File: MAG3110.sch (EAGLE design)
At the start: 4 parts

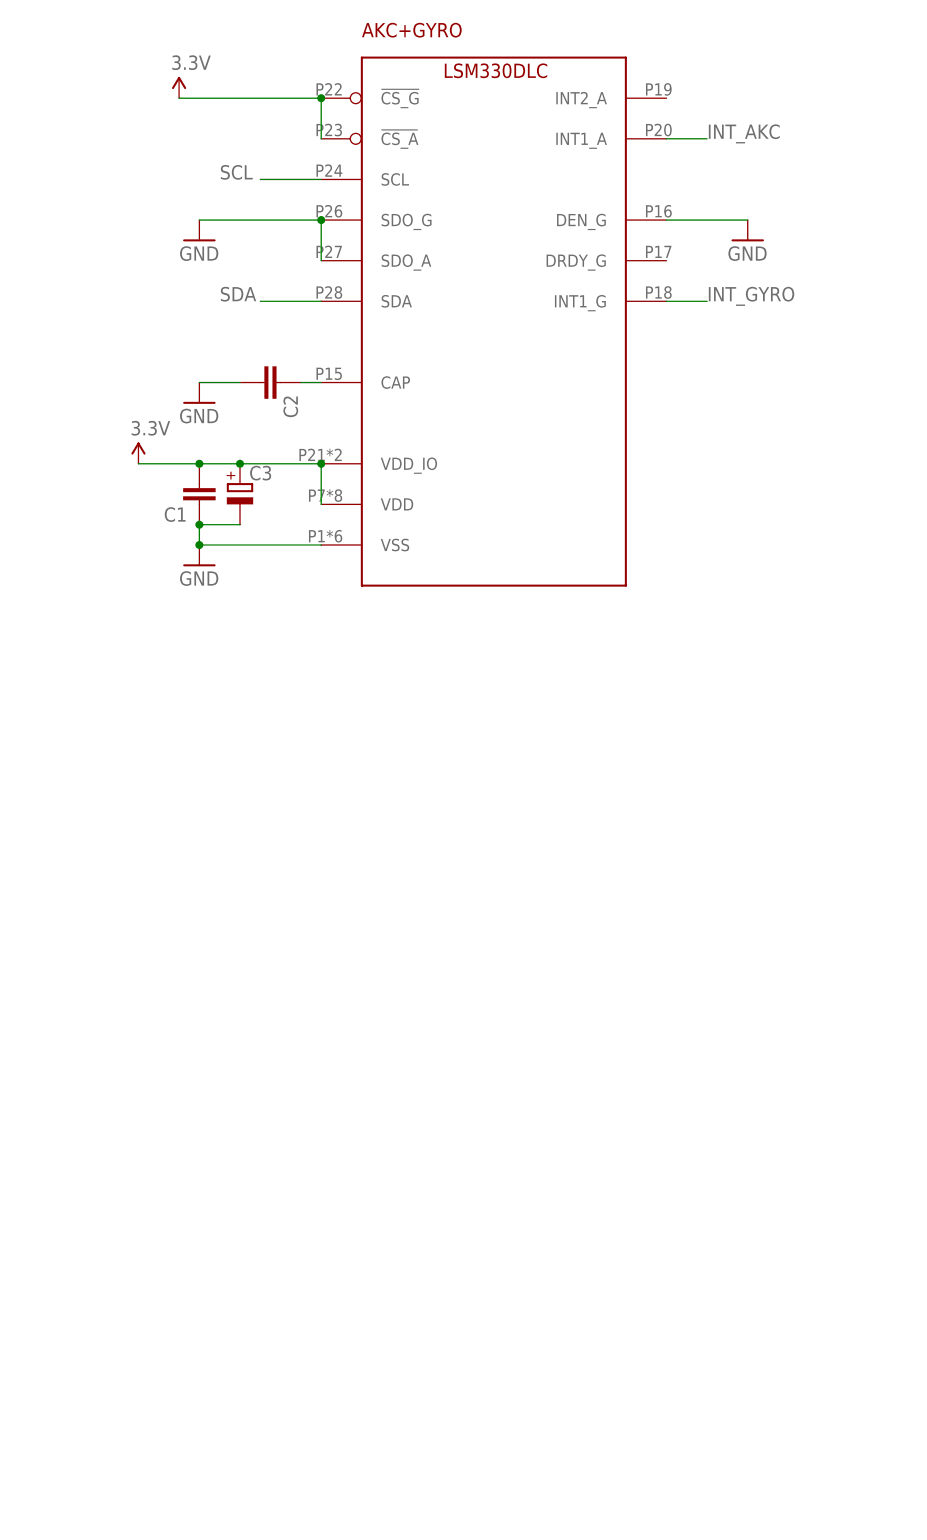
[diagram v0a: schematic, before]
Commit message: porzadki w plikach
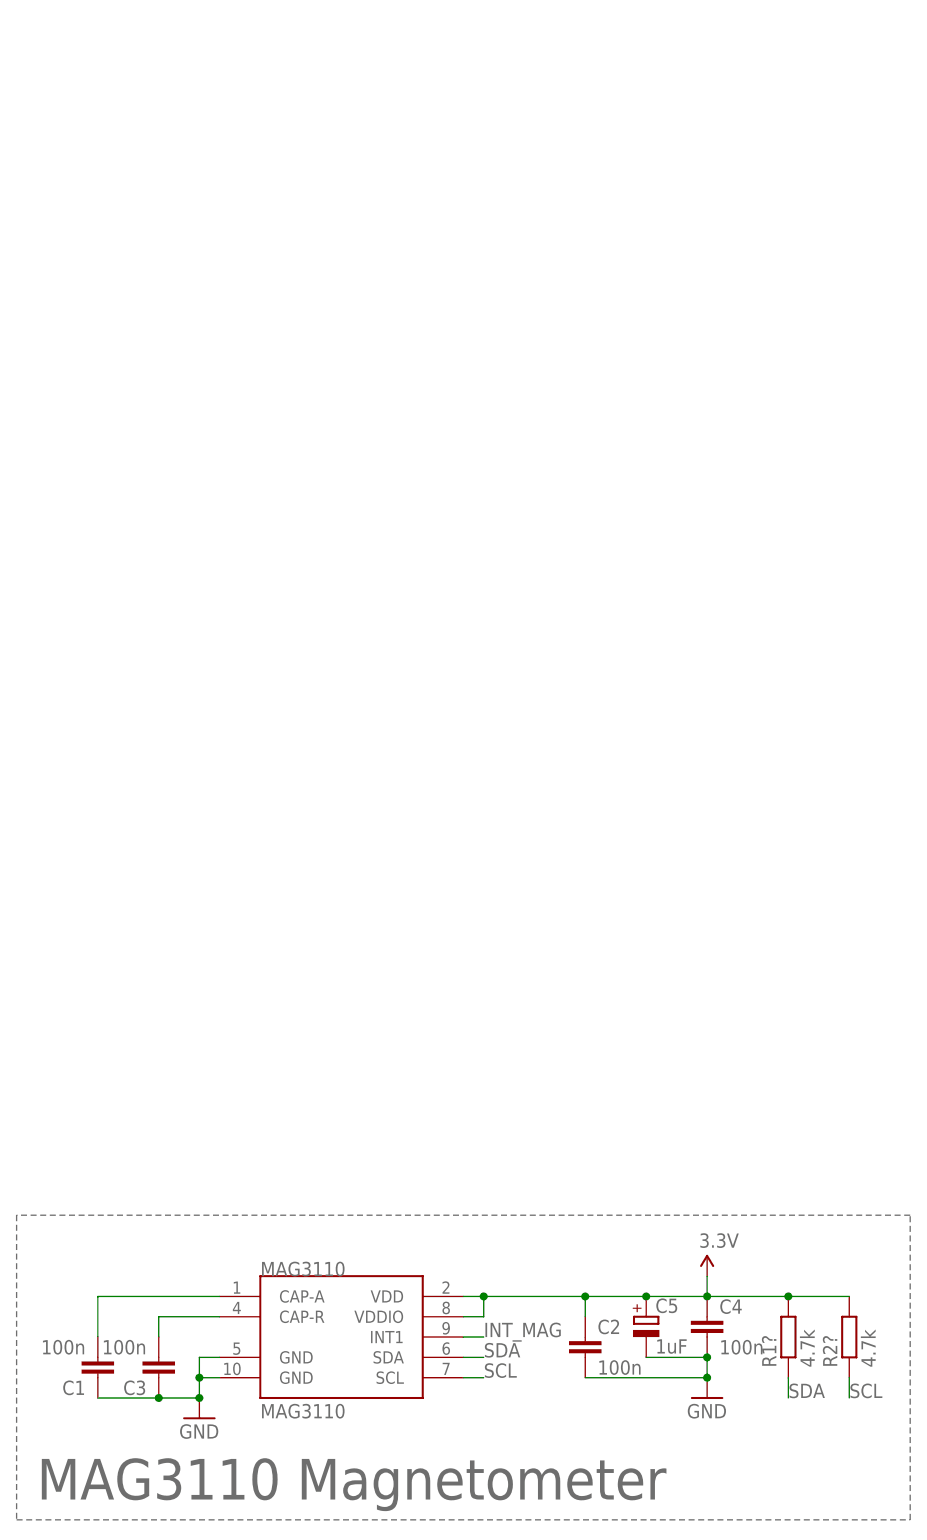
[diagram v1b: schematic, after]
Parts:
- removed AKC+GYRO: LSM330DLC, sensors-akc_zyr:LSM330DLC
- added C4: 100n, rcl:C-EUC0805
- added C5: 1uF, rcl:CPOL-EUSMCA
- added MAG3110: MAG3110, sparkfun-sensors (2):MAG3110
- added R1?, R2?: 4.7k, rcl:R-EU_R0805
- C1, C2: value (none) -> 100n; device resistor:C-EUC0805 -> rcl:C-EUC0805
- C3: value (none) -> 100n; device rcl:CPOL-EUSMCA -> rcl:C-EUC0805
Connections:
- removed net INT_AKC: AKC+GYRO.INT1_A
- removed net INT_GYRO: AKC+GYRO.INT1_G
- removed net N$1: AKC+GYRO.CAP, C2.1
- new net INT_MAG: MAG3110.INT1
- new net N$2: C3.2, MAG3110.CAP-R
- new net N$3: C1.2, MAG3110.CAP-A
- net 3.3V: now also C2.1, C4.1, C5.+, MAG3110.VDD, MAG3110.VDDIO, R1?.2, R2?.2; no longer AKC+GYRO.!CS_A, AKC+GYRO.!CS_G, AKC+GYRO.VDD, AKC+GYRO.VDD_IO, C1.2, C3.+
- net GND: now also C3.1, C4.2, C5.-, MAG3110.GND@10, MAG3110.GND@5; no longer AKC+GYRO.DEN_G, AKC+GYRO.SDO_A, AKC+GYRO.SDO_G, AKC+GYRO.VSS, C3.-
- net SCL: now also MAG3110.SCL, R2?.1; no longer AKC+GYRO.SCL
- net SDA: now also MAG3110.SDA, R1?.1; no longer AKC+GYRO.SDA
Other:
- note added: "MAG3110 Magnetometer"
- moved on the sheet: C1, C2
